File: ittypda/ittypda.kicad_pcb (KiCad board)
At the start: 2 copper layers, 132.5 x 67 mm, 161 parts, among them CN1 S2B-PH-SM4-TB, J1 USB_C_Receptacle_USB2.0_14P, J10 Solder Pad D+, J11 Solder Pad GND, J12 Solder Pad GND, J2 Conn_01x04_Pin, J3 Solder Pad D-, J4 Solder Pad D+, J5 Solder Pad 3.3V, J6 Solder Pad VBAT, J7 Solder Pad VBAT, J8 Solder Pad 3.3V, J9 Solder Pad D-, SW1 Switch, SW10 Switch, SW11 Switch, SW12 Switch, SW13 Switch, SW14 Switch, SW15 Switch, SW16 Switch, SW17 Switch, SW18 Switch, SW19 Switch, SW2 Switch, SW20 Switch, SW21 Switch, SW22 Switch, SW23 Switch, SW24 Switch, SW25 SLIDE SWITCH, SW26 Switch, SW27 Switch, SW28 Switch, SW29 Switch, SW3 Switch, SW30 Switch, SW31 Switch, SW32 Switch, SW33 Switch, SW34 Switch, SW36 Switch, SW37 Switch, SW38 Switch, SW39 Switch, SW4 Switch, SW41 Switch, SW42 Switch, SW43 Switch, SW44 Switch, SW45 Switch, SW46 Switch, SW47 Switch, SW48 Switch, SW49 Switch, SW5 Switch, SW50 Switch, SW51 Switch, SW52 Switch, SW53 Switch, SW54 Switch, SW55 Switch, SW56 Switch, SW57 Switch, SW58 Switch, SW59 Switch, SW6 Switch, SW60 Switch, SW61 Switch, SW7 Switch, SW8 Switch, SW9 Switch, U1 STM32F401RETx, U2 BQ24040DSQR, U3 TLV75801PDRV, Y1 16Mhz

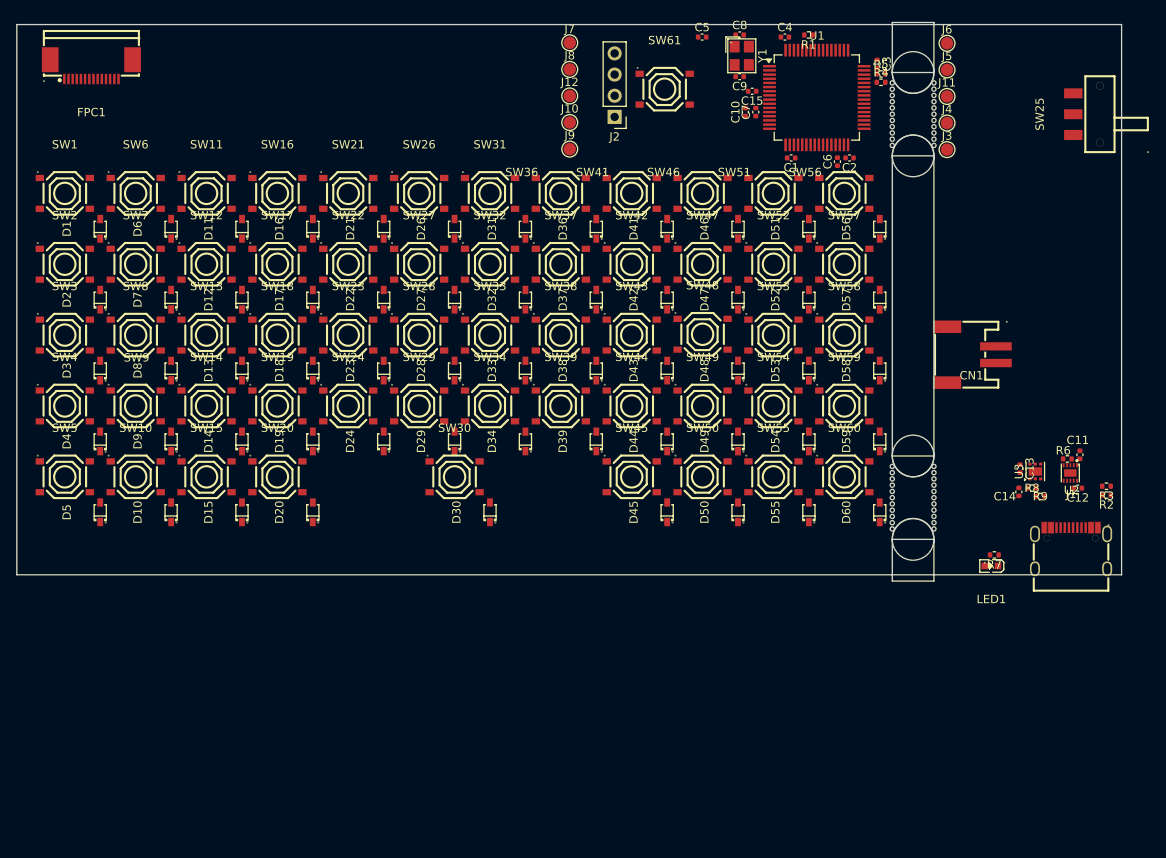
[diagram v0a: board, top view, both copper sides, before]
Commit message: move mousebites to bottom of pcb
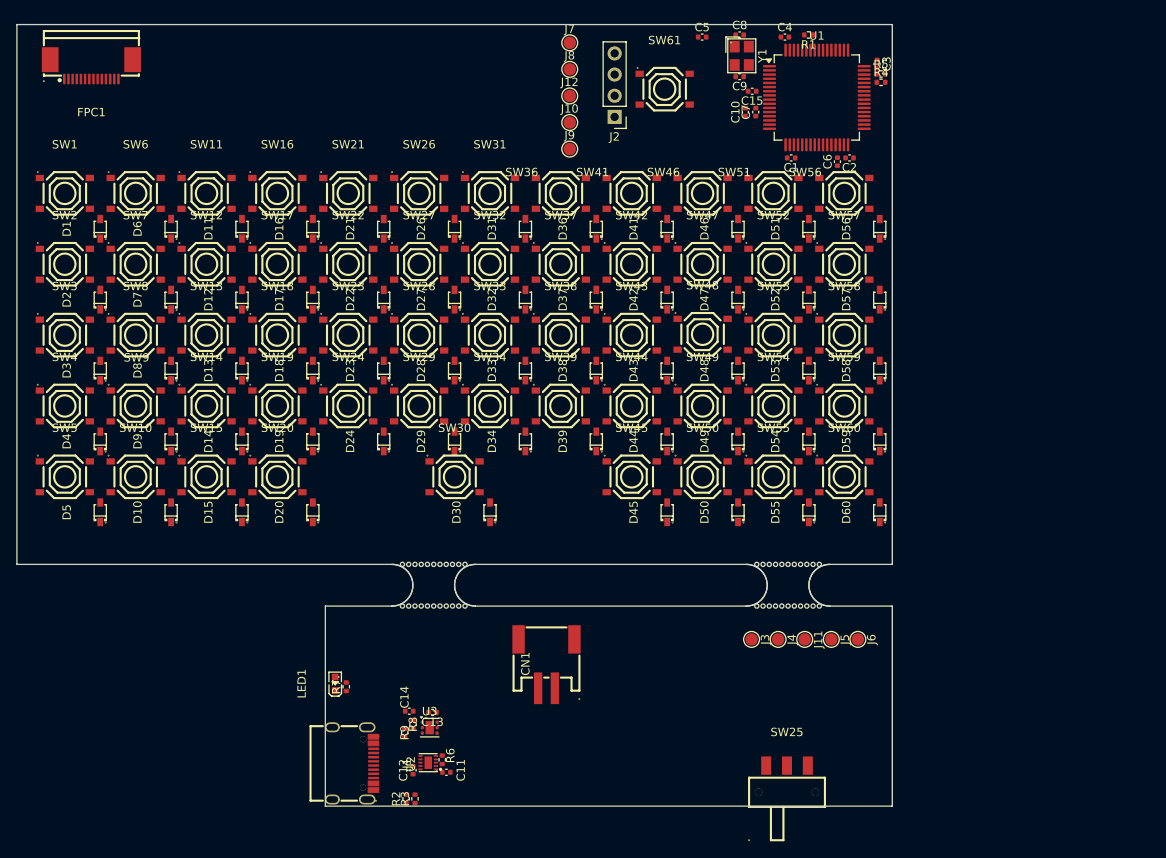
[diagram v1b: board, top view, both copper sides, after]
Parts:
- removed the mouse-bite-5mm-slot at (131.5, 41.5)
- removed the mouse-bite-5mm-slot at (131.5, 87.5)
- added mouse-bite-5mm-slot: VAL**, Panelization:mouse-bite-5mm-slot, F.Cu at (74.0, 98.0)
- added mouse-bite-5mm-slot: VAL**, Panelization:mouse-bite-5mm-slot, F.Cu at (116.5, 98.0)
- moved R2 91.6 mm to (70.7, 123.6), turned to 90 degrees
- moved R3 91.0 mm to (71.8, 123.6), turned to 90 degrees
- moved J1 89.9 mm to (64.3, 119.4), turned to -90 degrees
- moved C12 86.6 mm to (71.5, 120.2), turned to 90 degrees
- moved SW25 85.3 mm to (116.4, 119.6), turned to 0 degrees
- moved C11 85.0 mm to (75.5, 120.4), turned to 0 degrees
- moved U2 84.5 mm to (73.3, 119.3), turned to 90 degrees
- moved R6 83.2 mm to (75.0, 118.9), turned to -90 degrees
- moved R9 81.3 mm to (70.5, 115.7), turned to -90 degrees
- moved LED1 80.0 mm to (62.2, 109.8), turned to 90 degrees
- moved R8 79.5 mm to (71.5, 114.7), turned to -90 degrees
- moved R7 79.3 mm to (63.5, 110.2), turned to 90 degrees
- moved U3 78.9 mm to (73.5, 115.1), turned to 0 degrees
- moved C14 77.7 mm to (71.1, 113.1), turned to 180 degrees
- moved C13 76.3 mm to (73.9, 113.3), turned to 180 degrees
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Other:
- board size 132.5 x 67 mm -> 105 x 93.8 mm
